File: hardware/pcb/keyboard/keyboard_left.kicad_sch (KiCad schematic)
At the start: 31 parts, among them J1 SM03B-SRSS-TB, J2 PJ320D, J3 HRO_TYPE-C-31-M-12, J4 FH34SRJ-12S-0.5SH, SW29 PTS845, U3 PRTR5V0U2X, U4 XC6220B331MR-G, U5 STM32G431KBTx, Y1 8MHz 10pF

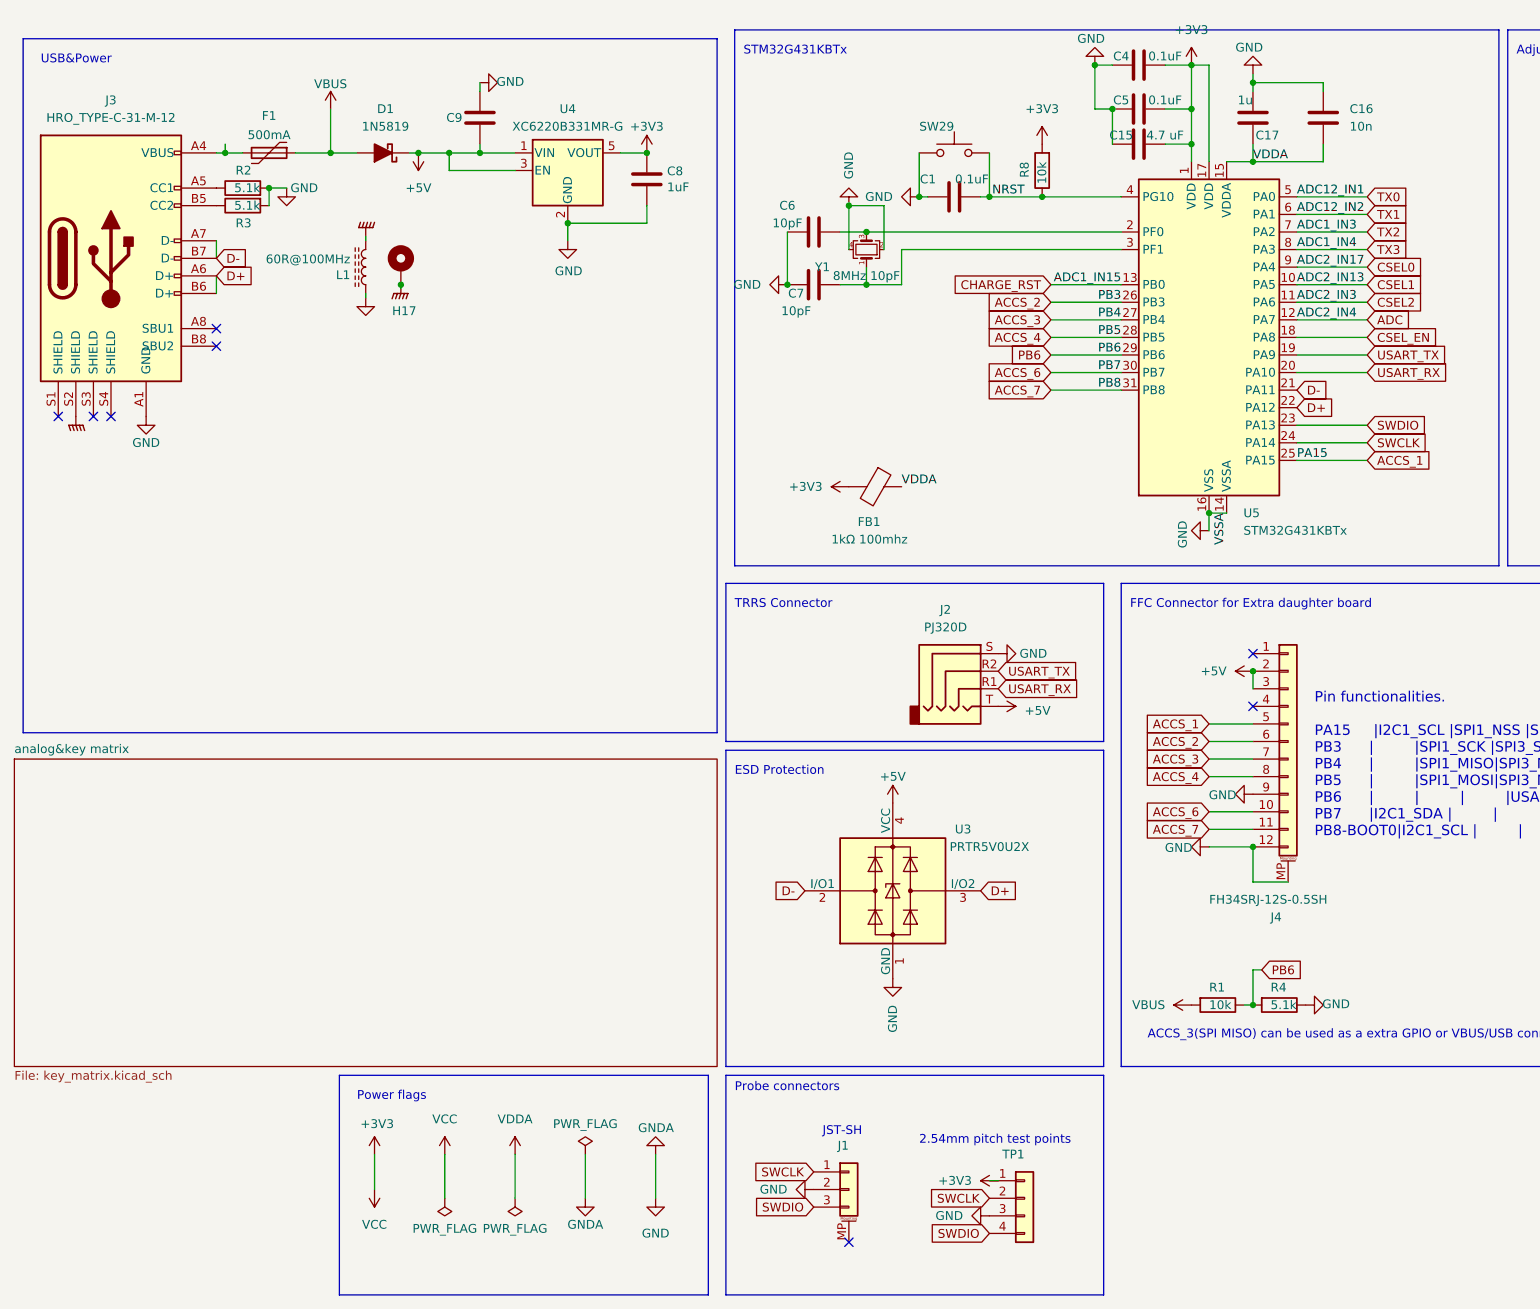
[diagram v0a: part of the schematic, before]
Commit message: init memory
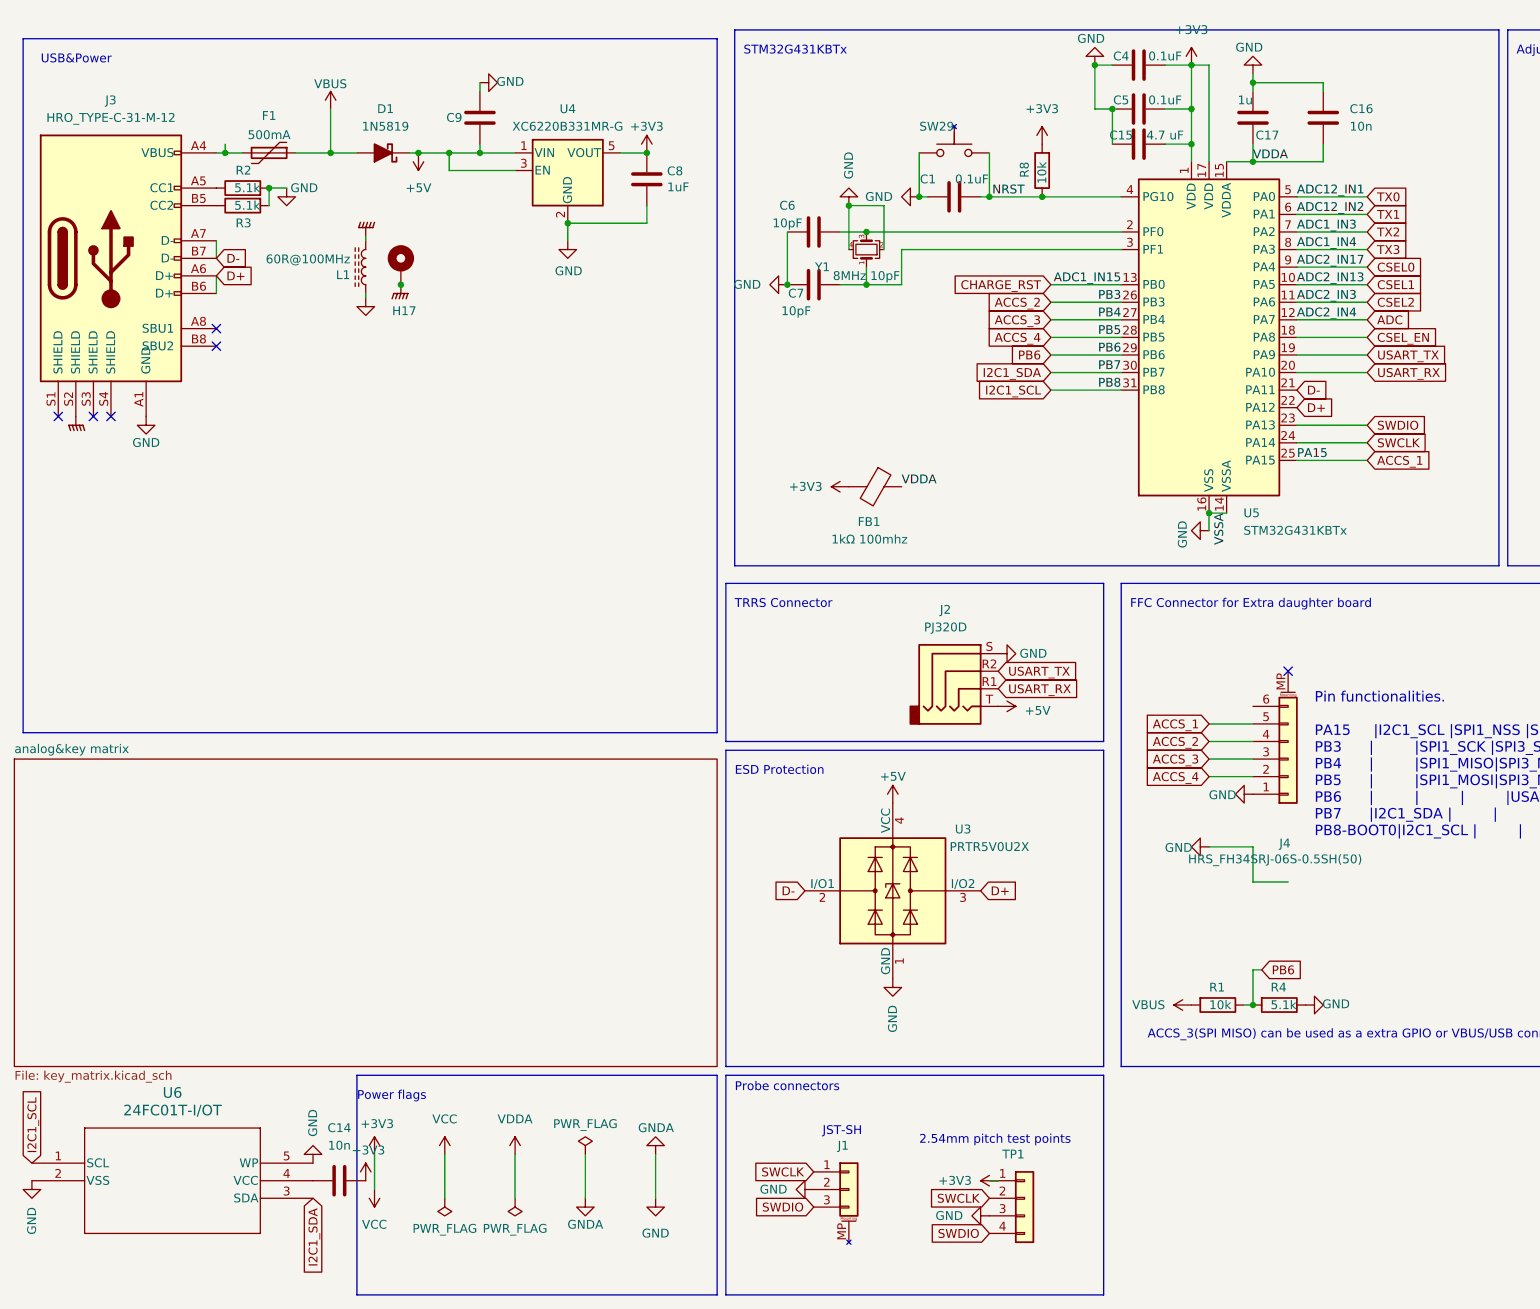
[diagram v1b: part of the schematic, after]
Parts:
- removed J4: FH34SRJ-12S-0.5SH, ec_parts:HRS_FH34SRJ-12S-0.5SH(50), symbol Connector_Generic_MountingPin:Conn_01x12_MountingPin
- added C14: 10n, PCM_Capacitor_SMD_AKL:C_0603_1608Metric, symbol Device:C
- added J4: HRS_FH34SRJ-06S-0.5SH(50), ec_parts:CONN6x1_FH34SRJ-6S-0.5SH50_HIR, symbol Connector_Generic_MountingPin:Conn_01x06_MountingPin
- added U6: 24FC01T-I/OT, SOT-23-5_2P9X1P6_MCH, symbol 24FC01T-I/OT:24FC01T-I_OT
- SW29: symbol Switch:SW_Push -> ec_parts:SW_Push
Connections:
- net +3V3: now also C14.1
- net ACCS_1: now also J4.5 (Pin_5)
- net ACCS_2: now also J4.4 (Pin_4)
- net ACCS_3: now also J4.3 (Pin_3)
- net ACCS_4: now also J4.2 (Pin_2)
- net GND: now also J4.1 (Pin_1), U6.2 (VSS), U6.5 (WP)
- net ACCS_6 renamed I2C1_SDA
- net I2C1_SDA: now also U6.3 (SDA)
- net ACCS_7 renamed I2C1_SCL
- net I2C1_SCL: now also U6.1 (SCL)
- new net: C14.2, U6.4 (VCC)
- no-connect marks 10 -> 8
